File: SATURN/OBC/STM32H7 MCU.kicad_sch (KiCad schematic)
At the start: 8 parts, among them IC1 STM32H735AGI6

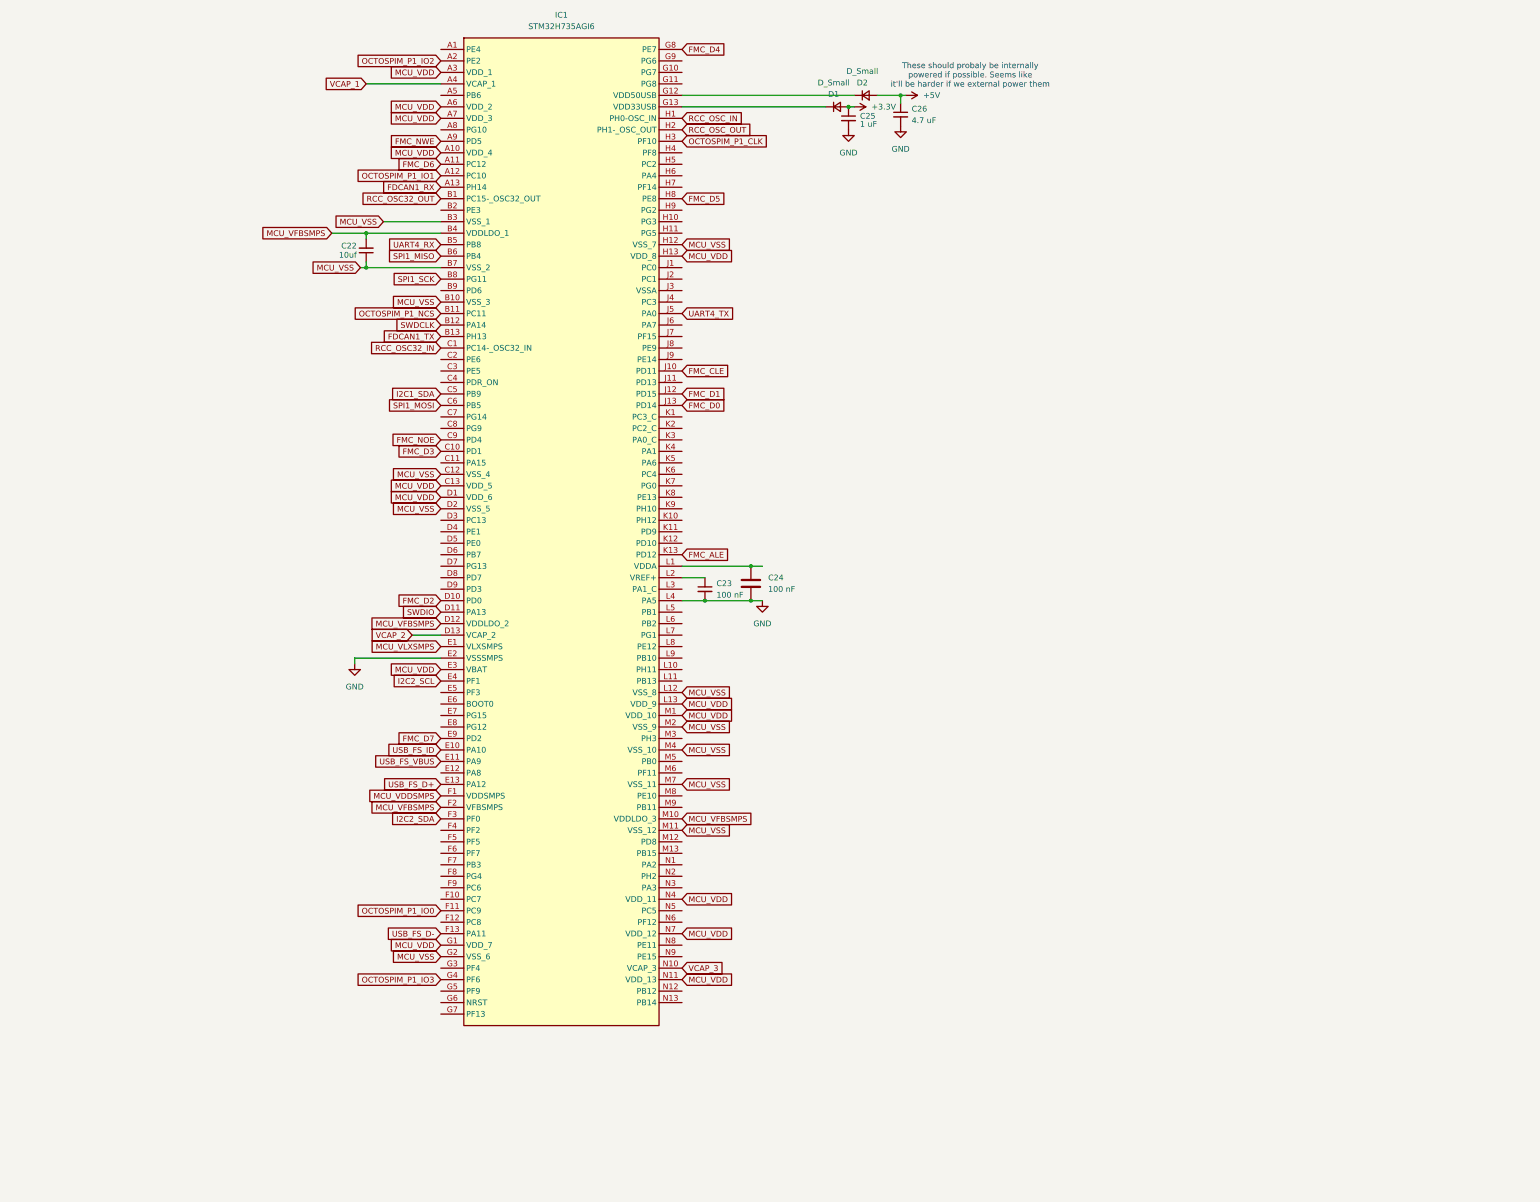
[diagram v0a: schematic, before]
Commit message: Buncha changes, had to merge manually, hopefully nothing is broken.
Added the second MCU
Updated USB switcher
Added backup battery to RTC
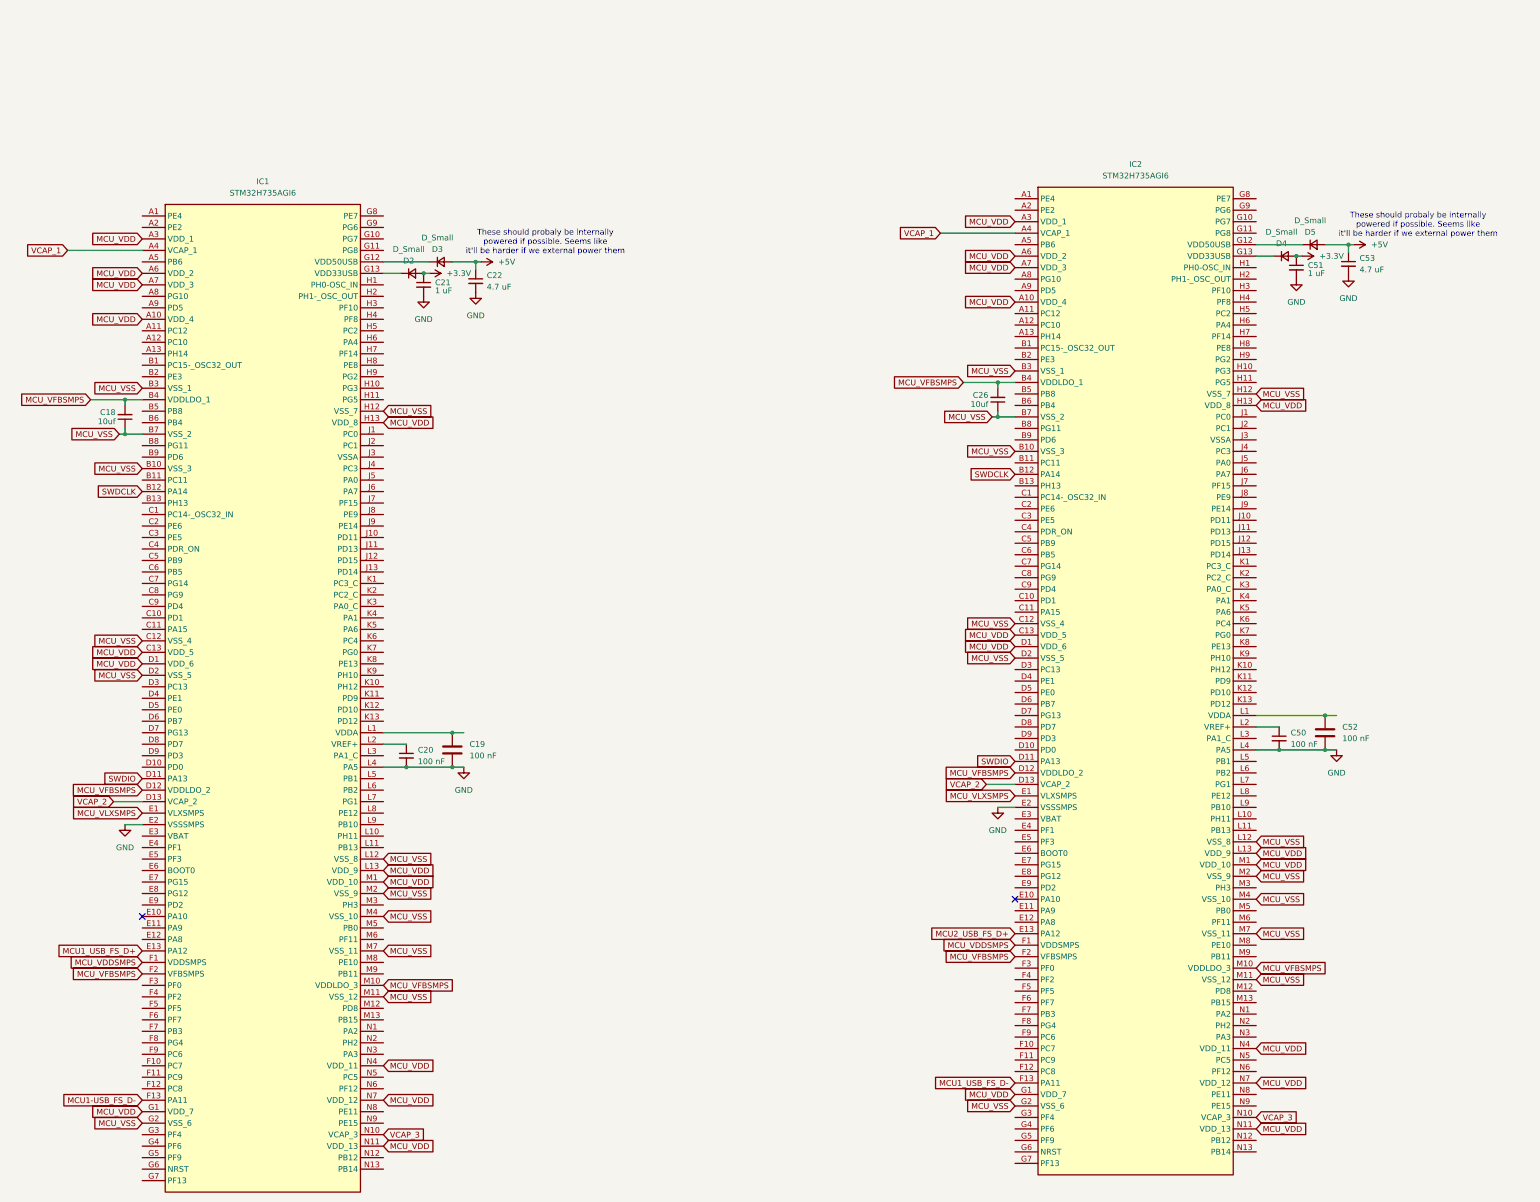
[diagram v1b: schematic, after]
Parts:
- removed C23: 100 nF, symbol Device:C_Small
- removed C24: 100 nF, symbol Device:C
- removed C25: 1 uF, symbol Device:C_Small
- removed D1: D_Small, symbol Device:D_Small
- added C18: 10uf, Capacitor_SMD:C_0603_1608Metric, symbol Device:C_Small
- added C19, C52: 100 nF, symbol Device:C
- added C20, C50: 100 nF, symbol Device:C_Small
- added C21, C51: 1 uF, symbol Device:C_Small
- added C53: 4.7 uF, symbol Device:C_Small
- added D3, D4, D5: D_Small, symbol Device:D_Small
- added IC2: STM32H735AGI6, Gabriel_footprints:BGA169C50P13X13_700X700X60, symbol STM32H735AGI6:STM32H735AGI6
- C22: value 10uf -> 4.7 uF; footprint Capacitor_SMD:C_0603_1608Metric -> (none)
- C26: value 4.7 uF -> 10uf; footprint (none) -> Capacitor_SMD:C_0603_1608Metric
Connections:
- net +3.3V: now also D2.2 (A), C21.1, C51.1, D4.2 (A)
- net +5V: now also C22.1, C53.1, D3.2 (A), D5.2 (A); no longer C26.1, D2.2 (A)
- net GND: now also C22.2, C19.2, C20.2, C21.2, C50.2, C51.2, C52.2, C53.2, IC2.E2 (VSSSMPS), IC2.L4 (PA5); no longer C26.2
- net MCU_VDD: now also IC2.A10 (VDD_4), IC2.A3 (VDD_1), IC2.A6 (VDD_2), IC2.A7 (VDD_3), IC2.C13 (VDD_5), IC2.D1 (VDD_6), IC2.G1 (VDD_7), IC2.H13 (VDD_8), IC2.L13 (VDD_9), IC2.M1 (VDD_10), IC2.N11 (VDD_13), IC2.N4 (VDD_11), IC2.N7 (VDD_12); no longer IC1.E3 (VBAT)
- net MCU_VDDSMPS: now also IC2.F1 (VDDSMPS)
- net MCU_VFBSMPS: now also C26.2, C18.2, IC2.B4 (VDDLDO_1), IC2.D12 (VDDLDO_2), IC2.F2 (VFBSMPS), IC2.M10 (VDDLDO_3); no longer C22.2
- net MCU_VLXSMPS: now also IC2.E1 (VLXSMPS)
- net MCU_VSS: now also C26.1, C18.1, IC2.B10 (VSS_3), IC2.B3 (VSS_1), IC2.B7 (VSS_2), IC2.C12 (VSS_4), IC2.D2 (VSS_5), IC2.G2 (VSS_6), IC2.H12 (VSS_7), IC2.L12 (VSS_8), IC2.M11 (VSS_12), IC2.M2 (VSS_9), IC2.M4 (VSS_10), IC2.M7 (VSS_11); no longer C22.1
- net SWDCLK: now also IC2.B12 (PA14)
- net SWDIO: now also IC2.D11 (PA13)
- net VCAP_1: now also IC2.A4 (VCAP_1)
- net VCAP_2: now also IC2.D13 (VCAP_2)
- net VCAP_3: now also IC2.N10 (VCAP_3)
- net at IC1.G13 (VDD33USB): now also D2.1 (K)
- net at IC1.G12 (VDD50USB): now also D3.1 (K); no longer D2.1 (K)
- net at IC1.L1 (VDDA): now also C19.1
- net at IC1.L2 (VREF+): now also C20.1
- net FDCAN1_RX: no longer names the net of IC1.A13 (PH14)
- net FDCAN1_TX: no longer names the net of IC1.B13 (PH13)
- net FMC_ALE: no longer names the net of IC1.K13 (PD12)
- net FMC_CLE: no longer names the net of IC1.J10 (PD11)
- net FMC_D0: no longer names the net of IC1.J13 (PD14)
- net FMC_D1: no longer names the net of IC1.J12 (PD15)
- net FMC_D2: no longer names the net of IC1.D10 (PD0)
- net FMC_D3: no longer names the net of IC1.C10 (PD1)
- net FMC_D4: no longer names the net of IC1.G8 (PE7)
- net FMC_D5: no longer names the net of IC1.H8 (PE8)
- net FMC_D6: no longer names the net of IC1.A11 (PC12)
- net FMC_D7: no longer names the net of IC1.E9 (PD2)
- net FMC_NOE: no longer names the net of IC1.C9 (PD4)
- net FMC_NWE: no longer names the net of IC1.A9 (PD5)
- net I2C1_SDA: no longer names the net of IC1.C5 (PB9)
- net I2C2_SCL: no longer names the net of IC1.E4 (PF1)
- net I2C2_SDA: no longer names the net of IC1.F3 (PF0)
- net OCTOSPIM_P1_CLK: no longer names the net of IC1.H3 (PF10)
- net OCTOSPIM_P1_IO0: no longer names the net of IC1.F11 (PC9)
- net OCTOSPIM_P1_IO1: no longer names the net of IC1.A12 (PC10)
- net OCTOSPIM_P1_IO2: no longer names the net of IC1.A2 (PE2)
- net OCTOSPIM_P1_IO3: no longer names the net of IC1.G4 (PF6)
- net OCTOSPIM_P1_NCS: no longer names the net of IC1.B11 (PC11)
- net RCC_OSC32_IN: no longer names the net of IC1.C1 (PC14-_OSC32_IN)
- net RCC_OSC32_OUT: no longer names the net of IC1.B1 (PC15-_OSC32_OUT)
- net RCC_OSC_IN: no longer names the net of IC1.H1 (PH0-OSC_IN)
- net RCC_OSC_OUT: no longer names the net of IC1.H2 (PH1-_OSC_OUT)
- net SPI1_MISO: no longer names the net of IC1.B6 (PB4)
- net SPI1_MOSI: no longer names the net of IC1.C6 (PB5)
- net SPI1_SCK: no longer names the net of IC1.B8 (PG11)
- net UART4_RX: no longer names the net of IC1.B5 (PB8)
- net UART4_TX: no longer names the net of IC1.J5 (PA0)
- net USB_FS_D+ renamed MCU1_USB_FS_D+
- net USB_FS_D- renamed MCU1-USB_FS_D-
- net USB_FS_ID: no longer names the net of IC1.E10 (PA10)
- net USB_FS_VBUS: no longer names the net of IC1.E11 (PA9)
- new net: D5.1 (K), IC2.G12 (VDD50USB)
- new net: D4.1 (K), IC2.G13 (VDD33USB)
- new net: C52.1, IC2.L1 (VDDA)
- new net: C50.1, IC2.L2 (VREF+)
- new net MCU1_USB_FS_D-: IC2.F13 (PA11)
- new net MCU2_USB_FS_D+: IC2.E13 (PA12)
- no-connect marks 0 -> 2
